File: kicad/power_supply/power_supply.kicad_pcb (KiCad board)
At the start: 2 copper layers, 71 x 99 mm, 46 parts, among them J1 Conn_WallSocket_Earth, J2 USB_C_Receptacle_USB2.0, J3 Conn_01x02, J4 Conn_02x08_Odd_Even, Q1 BCM53DS, Q2 BCM56DS, T1 70043K, U1 PCM2706CPJTR, Y1 12MHz±0.05%

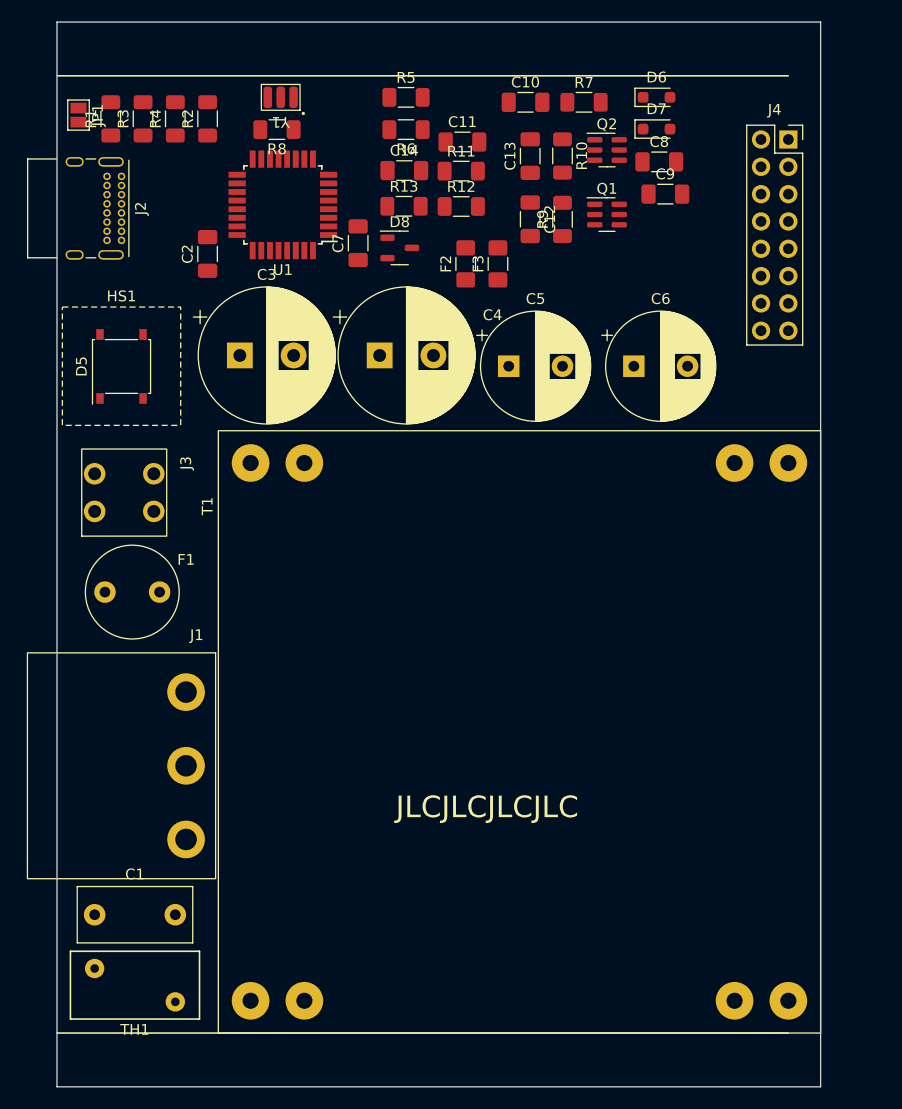
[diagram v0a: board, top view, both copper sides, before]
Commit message: commit
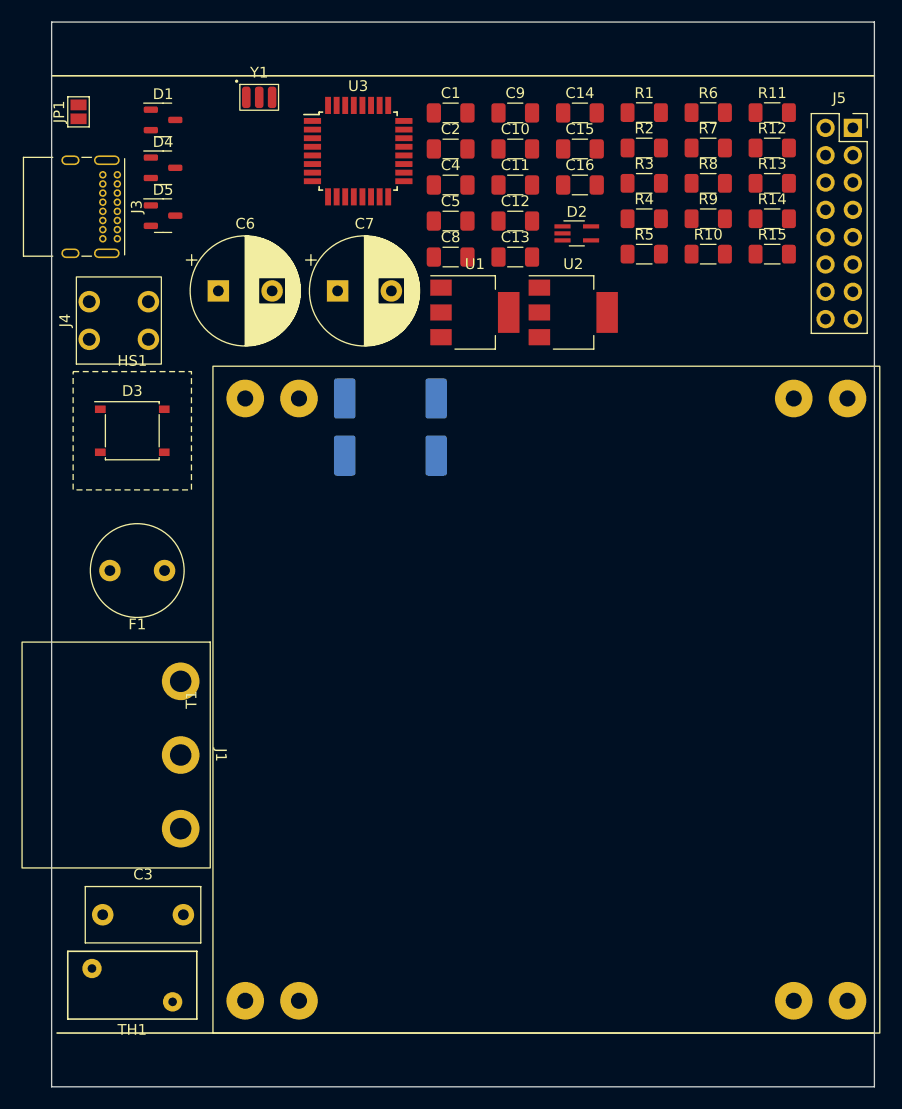
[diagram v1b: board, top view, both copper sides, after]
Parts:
- removed D6, D7: D, Diode_SMD:D_SOD-323_HandSoldering
- removed D8: ~, Package_TO_SOT_SMD:SOT-23-3
- removed J2: USB_C_Receptacle_USB2.0, Connector_USB:USB_C_Receptacle_GCT_USB4085
- removed Q1: BCM53DS, Package_SO:SC-74-6_1.5x2.9mm_P0.95mm
- removed Q2: BCM56DS, Package_SO:SC-74-6_1.5x2.9mm_P0.95mm
- added C15: 10u, Capacitor_SMD:C_1206_3216Metric_Pad1.33x1.80mm_HandSolder, F.Cu at (65.6, 25.8)
- added C16: 10u, Capacitor_SMD:C_1206_3216Metric_Pad1.33x1.80mm_HandSolder, F.Cu at (65.6, 29.1)
- added D1: ~, Package_TO_SOT_SMD:SOT-23-3, F.Cu at (26.9, 23.1)
- added D2: D_TVS_Quadruple, Package_TO_SOT_SMD:SOT-353_SC-70-5_Handsoldering, F.Cu at (65.3, 33.6)
- added D3: ~, Diode_SMD:Diode_Bridge_Vishay_MBLS, F.Cu at (24.0, 52.0)
- added D4: ~, Package_TO_SOT_SMD:SOT-23-3, F.Cu at (26.9, 27.6)
- added J5: Conn_02x08_Odd_Even, Connector_PinSocket_2.54mm:PinSocket_2x08_P2.54mm_Vertical, F.Cu at (91.0, 23.8)
- added R14: 1k1, Resistor_SMD:R_1206_3216Metric_Pad1.30x1.75mm_HandSolder, F.Cu at (83.5, 32.3)
- added R15: 100, Resistor_SMD:R_1206_3216Metric_Pad1.30x1.75mm_HandSolder, F.Cu at (83.5, 35.6)
- added U2: LM337_SOT223, Package_TO_SOT_SMD:SOT-223-3_TabPin2, F.Cu at (65.0, 41.0)
- added U3: PCM2706CPJTR, Package_QFP:TQFP-32_7x7mm_P0.8mm, F.Cu at (45.0, 26.0)
- C1: value 3n9 -> 100n; footprint Capacitor_THT:C_Disc_D10.5mm_W5.0mm_P7.50mm -> Capacitor_SMD:C_1206_3216Metric_Pad1.33x1.80mm_HandSolder
- C10, C13, C8: value 10u -> 100n
- C11, C9: value 100n -> 10u
- C2: value 1u -> 4n7
- C3: value 2m2 -> 3n9; footprint Capacitor_THT:CP_Radial_D12.5mm_P5.00mm -> Capacitor_THT:C_Disc_D10.5mm_W5.0mm_P7.50mm
- C4: value 2m2 -> 100n; footprint Capacitor_THT:CP_Radial_D12.5mm_P5.00mm -> Capacitor_SMD:C_1206_3216Metric_Pad1.33x1.80mm_HandSolder
- C5: value 470u -> 3u3; footprint Capacitor_THT:CP_Radial_D10.0mm_P5.00mm -> Capacitor_SMD:C_1206_3216Metric_Pad1.33x1.80mm_HandSolder
- C7: value 10u -> 470u; footprint Capacitor_SMD:C_1206_3216Metric_Pad1.33x1.80mm_HandSolder -> Capacitor_THT:CP_Radial_D10.0mm_P5.00mm
- D5: footprint Diode_SMD:Diode_Bridge_Vishay_MBLS -> Package_TO_SOT_SMD:SOT-23-3
- F2, F3: value 1A -> 500mA; footprint Fuse:Fuse_1206_3216Metric_Pad1.42x1.75mm_HandSolder -> Fuse:Fuse_Schurter_UMT250; moved to B.Cu
- J3: value Conn_01x02 -> USB_C_Receptacle_USB2.0; footprint library:WAGO_2086-11X2 -> Connector_USB:USB_C_Receptacle_GCT_USB4085
- J4: value Conn_02x08_Odd_Even -> Conn_01x02; footprint Connector_PinSocket_2.54mm:PinSocket_2x08_P2.54mm_Vertical -> library:WAGO_2086-11X2
- R1: value 5.1k -> 22
- R11: value 10k -> 1M
- R12: value 10k -> 100
- R13: value 16 -> 1k1
- R2: value 1k5 -> 33k
- R3, R4: value 22 -> 5k1
- R5: value 10k -> 1k5
- R6: value 10k -> 22
- R7: value 1k5 -> 22
- R8: value 1M -> 1k5
- T1: value 70043K -> 70063K; footprint library:Talema_Transformer_2P2S_10VA -> library:Talema_Transformer_2P2S_25VA
- U1: value PCM2706CPJTR -> LM317_SOT-223; footprint Package_QFP:TQFP-32_7x7mm_P0.8mm -> Package_TO_SOT_SMD:SOT-223-3_TabPin2
- moved C1 81.6 mm to (53.6, 22.4)
- moved J4 64.5 mm to (22.8, 41.8), turned to 90 degrees
- moved C3 53.5 mm to (21.2, 97.0)
- moved R1 49.6 mm to (71.6, 22.4), turned to 0 degrees
- moved R3 47.0 mm to (71.6, 29.0), turned to 0 degrees
- moved R4 44.6 mm to (71.6, 32.3), turned to 0 degrees
- moved R2 40.7 mm to (71.6, 25.7), turned to 0 degrees
- moved R8 40.4 mm to (77.5, 29.0), turned to 0 degrees
- moved C6 39.3 mm to (32.0, 39.0)
- moved R13 34.3 mm to (83.5, 29.0)
- moved J3 29.6 mm to (22.6, 28.2), turned to -90 degrees
- moved R11 29.4 mm to (83.5, 22.4)
- moved R12 29.4 mm to (83.5, 25.7)
- moved R6 28.1 mm to (77.5, 22.4), turned to 0 degrees
- moved R5 26.5 mm to (71.6, 35.6)
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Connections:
- C1 pad 1: Net-(J3-Pin_1) -> GND
- C1 pad 2: /NEUTRAL -> Net-(J1-EARTH)
- C10 pad 2: /VCOM -> Net-(U3-VCCP)
- C11 pad 1: GNDD -> Net-(D4-A)
- C11 pad 2: Net-(U1-VCCP) -> GND
- C12 pad 1: /CM+ -> GND
- C12 pad 2: GND -> Net-(D5-K)
- C13 pad 1: GND -> +20Vreg
- C13 pad 2: /CM- -> GND
- C14 pad 2: Net-(D8-A) -> -20Vreg
- C2 pad 1: GNDD -> Net-(D2-C)
- C2 pad 2: VBUS -> GNDD
- C3 pad 1: +25V -> Net-(J4-Pin_1)
- C3 pad 2: GND -> /NEUTRAL
- C4 pad 1: GND -> GNDD
- C4 pad 2: -25V -> VBUS
- C5 pad 1: +25V -> GNDD
- C5 pad 2: GND -> VBUS
- C6 pad 1: GND -> +25V
- C6 pad 2: -25V -> GND
- C7 pad 1: Net-(C7-Pad1) -> GND
- C7 pad 2: GND -> -25V
- C8 pad 1: GND -> GNDD
- C8 pad 2: Net-(C8-Pad2) -> +3V3
- C9 pad 2: +3V3 -> /VCOM
- D5 pad 1: /V_{rect}+ -> -25V
- D5 pad 2: /V_{tran}- -> -20Vreg
- D5 pad 3: /V_{rect}- -> Net-(D5-K)
- F1 pad 2: Net-(J3-Pin_1) -> Net-(J4-Pin_1)
- J1 pad 3: Net-(D8-A) -> Net-(J1-EARTH)
- J4 pad 1: +20Vreg -> Net-(J4-Pin_1)
- J4 pad 2: +25V -> /LIVE
- JP1 pad 2: Net-(J2-SHIELD) -> Net-(D2-C)
- R1 pad 1: Net-(J2-CC1) -> Net-(J1-EARTH)
- R1 pad 2: GNDD -> GND
- R10 pad 1: Net-(C8-Pad2) -> GND
- R11 pad 1: Net-(C7-Pad1) -> /XTI
- R11 pad 2: /CM+ -> /XTO
- R12 pad 1: Net-(C8-Pad2) -> +20Vreg
- R12 pad 2: /CM- -> Net-(D4-A)
- R13 pad 1: Net-(D8-A) -> Net-(D4-A)
- R2 pad 1: /CONN_D+ -> GNDD
- R2 pad 2: +3V3 -> Net-(D2-C)
- R3 pad 1: /CONN_D- -> Net-(J3-CC1)
- R3 pad 2: /D- -> GNDD
- R4 pad 1: /CONN_D+ -> Net-(J3-CC2)
- R4 pad 2: /D+ -> GNDD
- R5 pad 1: +25V -> /CONN_D+
- R5 pad 2: GND -> +3V3
- R6 pad 1: GND -> /CONN_D-
- R6 pad 2: -25V -> /D-
- R7 pad 1: /DT -> /CONN_D+
- R7 pad 2: +3V3 -> /D+
- R8 pad 1: /XTI -> /DT
- R8 pad 2: /XTO -> +3V3
- R9 pad 2: Net-(C7-Pad1) -> GND
- TH1 pad 1: Net-(J3-Pin_1) -> Net-(J4-Pin_1)
- U1 pad 1: GNDD -> Net-(D4-A)
- U1 pad 2: Net-(U1-VCCP) -> +20Vreg
- U1 pad 3: GNDD -> +25V
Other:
- board size 71 x 99 mm -> 76.5 x 99 mm
- board text added: "front face of front plate"
- board text removed: "1mm to panel PCB"
- board text removed: "JLCJLCJLCJLC"
